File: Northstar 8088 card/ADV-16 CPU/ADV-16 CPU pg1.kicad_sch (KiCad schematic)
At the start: 35 parts, among them J1 Power In, P1 northstar card edge, U11 74LS373, U12 8088-2, U13 74LS00, U14 74LS04, U16 74S08, U17 8284, U21 74LS153, U22 74LS74, U27 6309-1, U28 74LS373, U29 74LS245, U30 74LS244, U31 74LS10, U4 74S04, U42 74LS374, U43 74LS373, U44 74LS138, U5 74LS32, U8 74LS74, Y1 24MHz

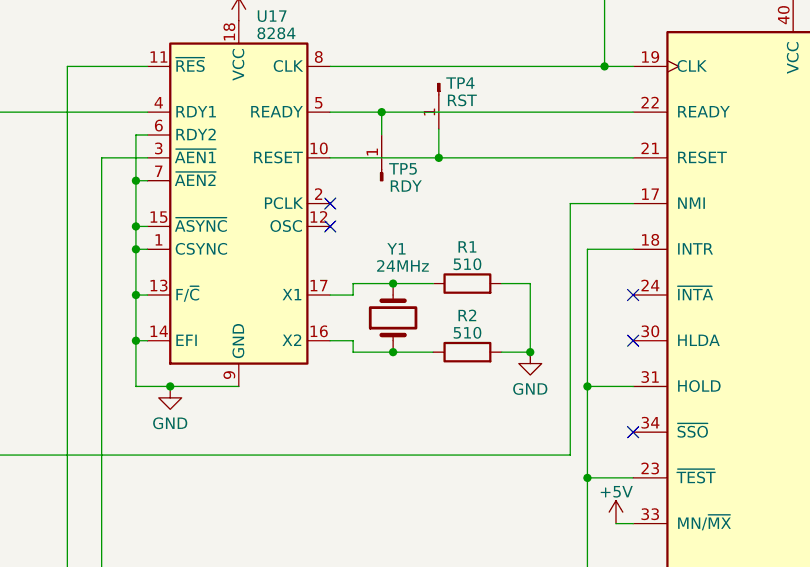
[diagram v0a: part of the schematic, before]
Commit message: more routing
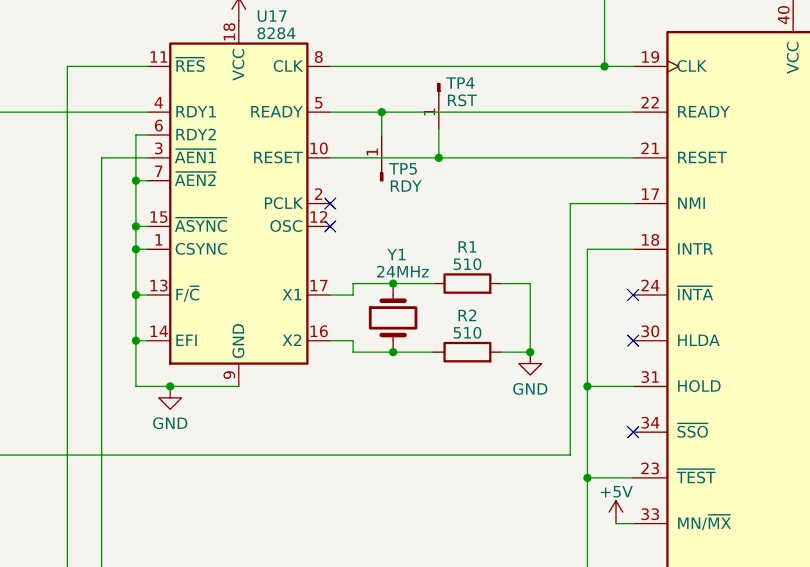
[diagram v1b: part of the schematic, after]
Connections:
- net at R2.1, U17.16 (X2): now also Y1.2; no longer Y1.1
- net at R1.1, U17.17 (X1): now also Y1.1; no longer Y1.2
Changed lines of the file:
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@@
         )
         (path "/a752c0c4-4fb2-47b8-9f01-e1cc48260014/6961fefb-6c96-4f21-a457-cfd11df00fb0"
-          (reference "R1") (unit 1)
+          (reference "R2") (unit 1)
         )
       )
@@
         )
         (path "/a752c0c4-4fb2-47b8-9f01-e1cc48260014/6961fefb-6c96-4f21-a457-cfd11df00fb0"
-          (reference "R2") (unit 1)
+          (reference "R1") (unit 1)
         )
       )
@@
     )
   )
-  (symbol (lib_id "Device:Crystal") (at 74.295 135.255 90) (unit 1)
+  (symbol (lib_id "Device:Crystal") (at 74.295 135.255 90) (mirror x) (unit 1)
     (in_bom yes) (on_board yes) (dnp no)
-    (property "Reference" "Y1" (at 73.66 127.635 90)
+    (property "Reference" "Y1" (at 73.66 128.27 90)
       (effects (font (size 1.27 1.27)) (justify right))
     )
-    (property "Value" "24MHz" (at 72.39 129.54 90)
+    (property "Value" "24MHz" (at 72.39 130.175 90)
       (effects (font (size 1.27 1.27)) (justify right))
     )
